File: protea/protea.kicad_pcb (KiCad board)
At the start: 2 copper layers, 92 x 44 mm, 72 parts, among them J1 USB4215-03-A, J2 D-SUB 9 Male, J3 676430910, J4 HDMI Female, J5 ESP8266 Prog, J6 SD04H0SB, U1 NCP1117 3.3, U2 W25Q128JVSIQ, U3 RP2040, U4 MAX232CSE+, U5 ESP8266-12E_ESP-12E, Y1 12 MHz

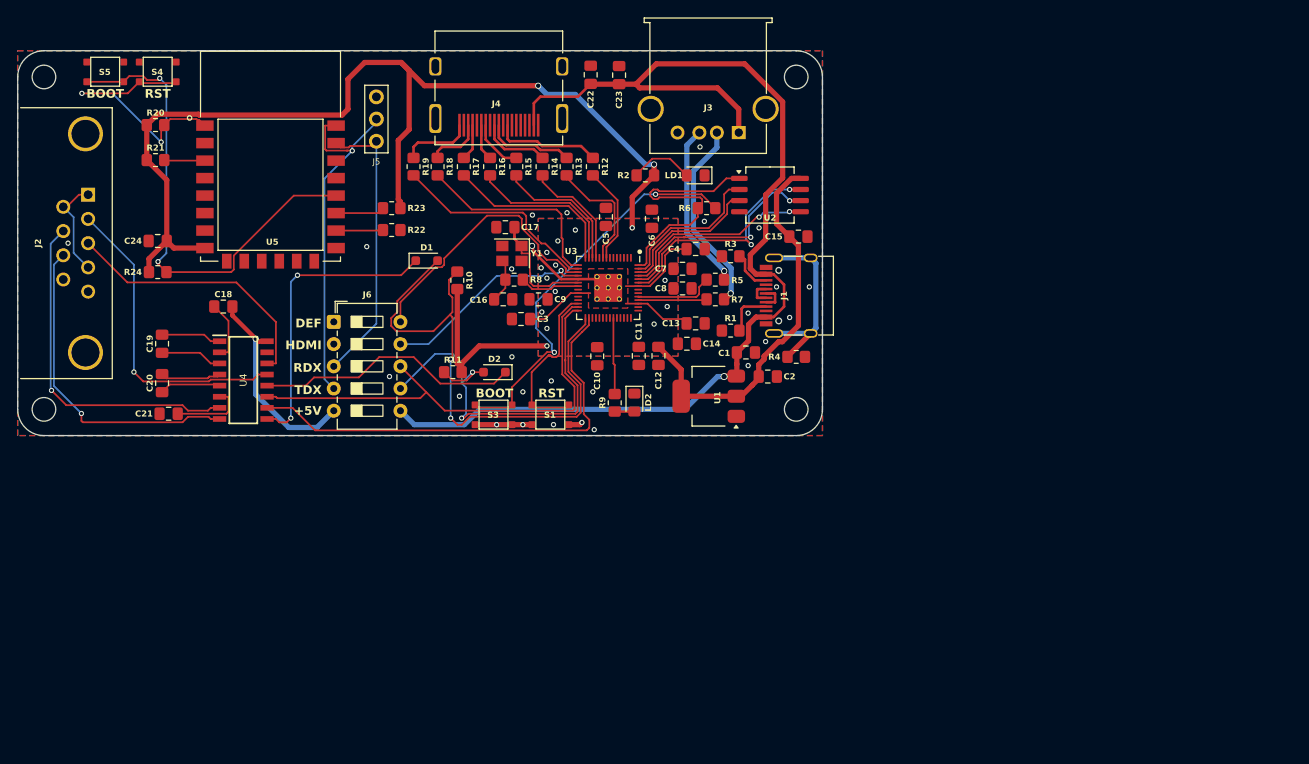
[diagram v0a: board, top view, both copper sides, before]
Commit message: Protea 1.1 WIP
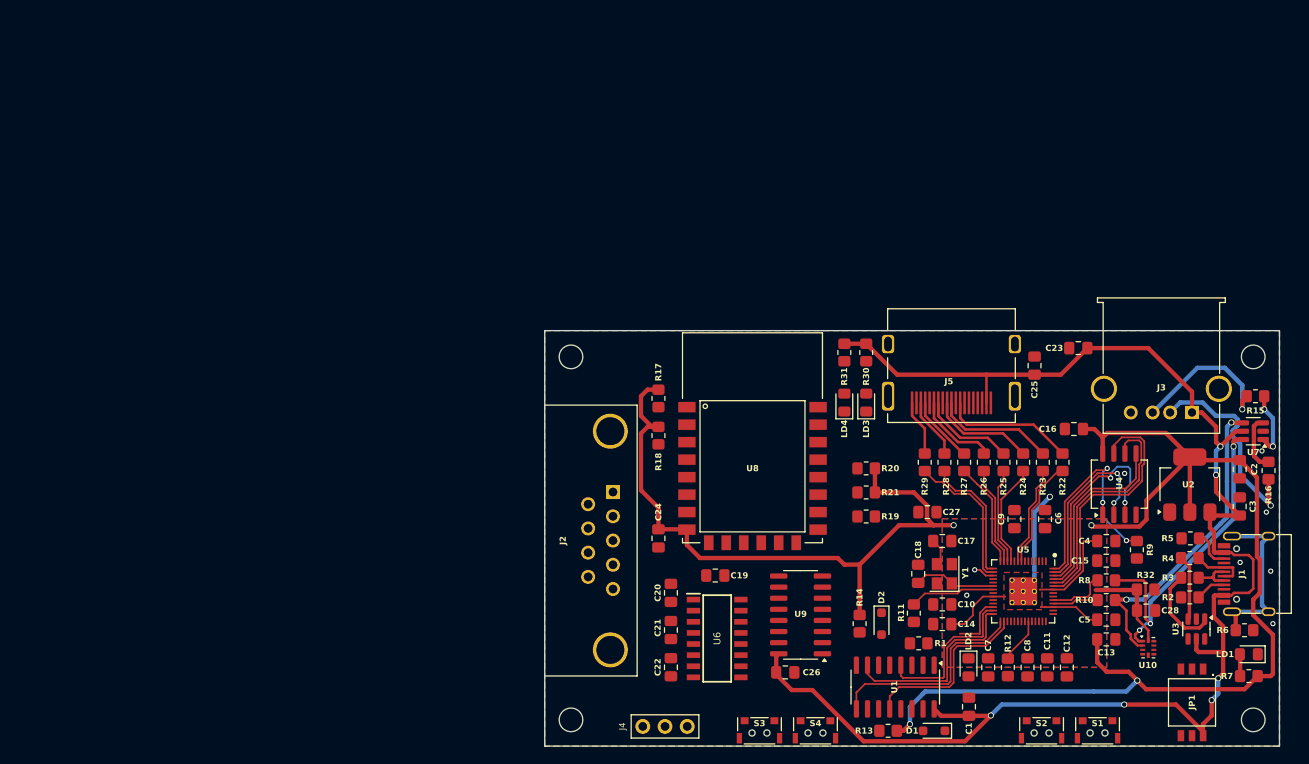
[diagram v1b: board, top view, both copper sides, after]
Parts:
- removed J6: SD04H0SB, FRANK:DIP Switch (5x5)
- removed S5: Flash, FRANK:Button (SMD, 3x3mm, 1-1)
- added C25: 100n, FRANK:Capacitor (0805), F.Cu at (193.8, 59.0)
- added C26: 100n, FRANK:Capacitor (0805), F.Cu at (165.2, 94.1)
- added C27: 100n, FRANK:Capacitor (0805), F.Cu at (181.5, 75.8)
- added C28: 100n, FRANK:Capacitor (0805), F.Cu at (206.5, 87.0)
- added JP1: Main Jumpers, FRANK:DS05127203BKSMTTR, F.Cu at (211.8, 97.5)
- added LD3: TX, FRANK:LED (0805), F.Cu at (174.5, 63.2)
- added LD4: RX, FRANK:LED (0805), F.Cu at (172.0, 63.2)
- added R25: 270R, FRANK:Resistor (0805), F.Cu at (190.2, 70.1)
- added R26: 270R, FRANK:Resistor (0805), F.Cu at (187.9, 70.1)
- added R27: 270R, FRANK:Resistor (0805), F.Cu at (185.7, 70.1)
- added R28: 270R, FRANK:Resistor (0805), F.Cu at (183.4, 70.1)
- added R29: 270R, FRANK:Resistor (0805), F.Cu at (181.2, 70.1)
- added R30: 1.5K, FRANK:Resistor (0805), F.Cu at (174.5, 57.5)
- added R31: 1.5K, FRANK:Resistor (0805), F.Cu at (172.0, 57.5)
- added R32: 10K, FRANK:Resistor (0805), F.Cu at (206.4, 84.6)
- added S2: Reset, FRANK:TACT-SIDE-4623, F.Cu at (194.6, 101.0)
- added U10: TS3USB221RSER, FRANK:UQFN-10, F.Cu at (206.8, 91.2)
- added U6: MAX232CSE+, FRANK:SOIC127P600X175-16N, F.Cu at (157.5, 90.2)
- added U7: USBLC6-2SC6, FRANK:SOT-23-6, F.Cu at (218.8, 66.5)
- added U8: ESP8266-12E_ESP-12E, FRANK:ESP8266 ESP-12E, F.Cu at (161.5, 70.8)
- added U9: CH340C, FRANK:SOP-16, F.Cu at (167.0, 87.5)
- C1: value 10u -> 100n
- C13: value 1u -> 100n
- C15: value 100n -> 1u
- C16: value 15p -> 100n
- C18: value 1u -> 15p
- C22: value 10u -> 1u
- C23, C3: value 100n -> 10u
- J4: value HDMI Female -> ESP8266 Prog; footprint FRANK:HDMI (female) -> FRANK:Pin Header (1x03)
- J5: value ESP8266 Prog -> HDMI Female; footprint FRANK:Pin Header (1x03) -> FRANK:HDMI (female)
- LD1: value Green -> Power
- R1: value 5.1K -> 10K
- R10, R8: value 1K -> 27R
- R12, R13, R14: value 270R -> 1K
- R15, R16: value 270R -> 22R
- R17, R18, R19: value 270R -> 10K
- R2: value 1K -> 5.1K
- R22, R23, R24: value 10K -> 270R
- R3: value 5.1K -> 22R
- R4: value 1M -> 22R
- R5: value 27R -> 5.1K
- R6: value 1K -> 1M
- R7: value 27R -> 1K
- S1: value Reset -> Boot; footprint FRANK:Button (SMD, 3x3mm, 1-1) -> FRANK:TACT-SIDE-4623
- S3: value Boot -> Reset; footprint FRANK:Button (SMD, 3x3mm, 1-1) -> FRANK:TACT-SIDE-4623
- S4: value Reset -> Flash; footprint FRANK:Button (SMD, 3x3mm, 1-1) -> FRANK:TACT-SIDE-4623
- U1: value NCP1117 3.3 -> SN74CBT3257CDR; footprint FRANK:SOT-223 -> FRANK:SOP-16
- U2: value W25Q128JVSIQ -> NCP1117 3.3; footprint FRANK:SOIC-8 -> FRANK:SOT-223
- U3: value RP2040 -> USBLC6-2SC6; footprint FRANK:QFN 56 -> FRANK:SOT-23-6
- U4: value MAX232CSE+ -> W25Q128JVSIQ; footprint FRANK:SOIC127P600X175-16N -> FRANK:SOIC-8
- U5: value ESP8266-12E_ESP-12E -> RP2040; footprint FRANK:ESP8266 ESP-12E -> FRANK:QFN 56
- moved H2 141.9 mm to (218.8, 58.0)
- moved S4 109.0 mm to (168.7, 101.0), turned to 180 degrees
- moved R24 101.3 mm to (192.4, 70.1), turned to -90 degrees
- moved U4 100.9 mm to (203.4, 72.6), turned to 90 degrees
- moved U5 97.7 mm to (192.4, 84.8), turned to -90 degrees
- moved R16 95.5 mm to (220.5, 71.0)
- moved R20 90.2 mm to (174.5, 70.8), turned to 180 degrees
- moved R21 89.7 mm to (174.5, 73.5), turned to 180 degrees
- moved R15 88.5 mm to (219.0, 62.5), turned to 180 degrees
- moved C18 85.1 mm to (180.4, 82.8), turned to 90 degrees
- moved C3 84.9 mm to (217.2, 75.1), turned to 90 degrees
- moved LD1 83.7 mm to (218.2, 92.0)
- moved R10 82.7 mm to (201.9, 85.8), turned to 180 degrees
- moved R22 81.2 mm to (196.9, 70.1), turned to -90 degrees
- moved R23 79.9 mm to (194.7, 70.1), turned to -90 degrees
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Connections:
- C1 pad 1: VBUS -> GND
- C1 pad 2: GND -> VBUS
- C13 pad 1: Net-(U3-VREG_VOUT) -> +3V3
- C14 pad 1: +3V3 -> Net-(U5-VREG_VOUT)
- C16 pad 1: Net-(C16-Pad1) -> +3V3
- C17 pad 1: /RP2040/XIN -> Net-(C17-Pad1)
- C18 pad 1: /RS232/V+ -> /RP2040/XIN
- C18 pad 2: /RS232_VBUS -> GND
- C19 pad 1: /RS232/C1- -> /RS232/V+
- C19 pad 2: /RS232/C1+ -> /RS232_VBUS
- C20 pad 1: /RS232/C2- -> /RS232/C1-
- C20 pad 2: /RS232/C2+ -> /RS232/C1+
- C21 pad 1: /RS232/V- -> /RS232/C2-
- C21 pad 2: GND -> /RS232/C2+
- C22 pad 1: GND -> /RS232/V-
- C22 pad 2: VBUS -> GND
- C23 pad 1: VBUS -> GND
- C23 pad 2: GND -> VBUS
- C3 pad 1: Net-(U3-VREG_VOUT) -> VBUS
- C4 pad 1: Net-(U3-VREG_VOUT) -> Net-(U5-VREG_VOUT)
- C5 pad 1: +3V3 -> Net-(U5-VREG_VOUT)
- D1 pad 2: /GPIO18 -> /RS232_CTS
- D2 pad 2: /GPIO17 -> /RS232_RX
- J1 pad 5: /Power/D- -> Net-(J1-DN1)
- J1 pad 6: /Power/D+ -> Net-(J1-DP1)
- J1 pad 7: /Power/D- -> Net-(J1-DN1)
- J1 pad 8: /Power/D+ -> Net-(J1-DP1)
- J3 pad 2: /D- -> Net-(J3-D-)
- J3 pad 3: /D+ -> Net-(J3-D+)
- J4 pad 1: Net-(J4-D2P) -> /ESP_RXD
- J4 pad 2: GND -> /ESP_TXD
- J4 pad 3: Net-(J4-D2N) -> GND
- J5 pad 1: /ESP_RXD -> Net-(J5-D2P)
- J5 pad 2: /ESP_TXD -> GND
- J5 pad 3: GND -> Net-(J5-D2N)
- R1 pad 2: Net-(J1-CC1) -> /SN74_S
- R10 pad 1: /GPIO18 -> /RP_D-
- R10 pad 2: +3V3 -> Net-(U5-USB_DM)
- R11 pad 1: /GPIO17 -> /RP2040/XOUT
- R11 pad 2: +3V3 -> Net-(C17-Pad1)
- R12 pad 1: Net-(J4-CLKN) -> Net-(LD2-A)
- R12 pad 2: /GPIO6 -> /RP2040/GPIO25
- R13 pad 1: Net-(J4-CLKP) -> /RS232_CTS
- R13 pad 2: /GPIO7 -> +3V3
- R14 pad 1: Net-(J4-D0N) -> /RS232_RX
- R14 pad 2: /GPIO8 -> +3V3
- R15 pad 1: Net-(J4-D0P) -> Net-(R15-Pad1)
- R15 pad 2: /GPIO9 -> Net-(J3-D+)
- R16 pad 1: Net-(J4-D1N) -> Net-(R16-Pad1)
- R16 pad 2: /GPIO10 -> Net-(J3-D-)
- R17 pad 1: Net-(J4-D1P) -> +3V3
- R17 pad 2: /GPIO11 -> Net-(U8-RESET)
- R18 pad 1: Net-(J4-D2N) -> +3V3
- R18 pad 2: /GPIO12 -> Net-(U8-EN)
- R19 pad 1: Net-(J4-D2P) -> GND
- R19 pad 2: /GPIO13 -> Net-(U8-IO15)
- R2 pad 1: Net-(LD1-A) -> GND
- R2 pad 2: +3V3 -> Net-(J1-CC1)
- R20 pad 2: Net-(U5-RESET) -> Net-(U8-IO0)
- R21 pad 2: Net-(U5-EN) -> Net-(U8-IO2)
- R22 pad 1: GND -> Net-(J5-CLKN)
- R22 pad 2: Net-(U5-IO15) -> /GPIO6
- R23 pad 1: +3V3 -> Net-(J5-CLKP)
- R23 pad 2: Net-(U5-IO2) -> /GPIO7
- R24 pad 1: +3V3 -> Net-(J5-D0N)
- R24 pad 2: Net-(U5-IO0) -> /GPIO8
- R3 pad 1: GND -> Net-(R3-Pad1)
- R3 pad 2: Net-(J1-CC2) -> Net-(J1-DN1)
- R4 pad 1: Net-(J1-SHIELD) -> Net-(R4-Pad1)
- R4 pad 2: GND -> Net-(J1-DP1)
- R5 pad 1: /D+ -> GND
- R5 pad 2: Net-(U3-USB_DP) -> Net-(J1-CC2)
- R6 pad 1: /RP2040/QSPI_SS -> Net-(J1-SHIELD)
- R6 pad 2: Net-(R6-Pad2) -> GND
- R7 pad 1: /D- -> Net-(LD1-A)
- R7 pad 2: Net-(U3-USB_DM) -> +3V3
- R8 pad 1: /RP2040/XOUT -> /RP_D+
- R8 pad 2: Net-(C16-Pad1) -> Net-(U5-USB_DP)
- R9 pad 1: Net-(LD2-A) -> /RP2040/QSPI_SS
- R9 pad 2: /RP2040/GPIO25 -> Net-(R9-Pad2)
- S1 pad 1: /RUN -> Net-(R9-Pad2)
- S3 pad 1: Net-(R6-Pad2) -> GND
- S3 pad 2: GND -> Net-(U8-RESET)
- S4 pad 2: Net-(U5-RESET) -> Net-(U8-IO0)
- U1 pad 1: GND -> /SN74_S
- U1 pad 2: +3V3 -> /ESP_RXD
- U1 pad 3: VBUS -> /RS232_TX
- U2 pad 1: /RP2040/QSPI_SS -> GND
- U2 pad 2: /RP2040/QSPI_SD1 -> +3V3
- U2 pad 3: /RP2040/QSPI_SD2 -> VBUS
- U3 pad 1: +3V3 -> Net-(R3-Pad1)
- U3 pad 2: /GPIO0 -> GND
- U3 pad 3: /GPIO1 -> Net-(R4-Pad1)
- U3 pad 4: /GPIO2 -> /PW_D+
- U3 pad 5: /GPIO3 -> VBUS
- U3 pad 6: /GPIO4 -> /PW_D-
- U4 pad 1: /RS232/C1+ -> /RP2040/QSPI_SS
- U4 pad 2: /RS232/V+ -> /RP2040/QSPI_SD1
- U4 pad 3: /RS232/C1- -> /RP2040/QSPI_SD2
- U4 pad 4: /RS232/C2+ -> GND
- U4 pad 5: /RS232/C2- -> /RP2040/QSPI_SD0
- U4 pad 6: /RS232/V- -> /RP2040/QSPI_SCLK
- U4 pad 7: /RS232/CTS_IN -> /RP2040/QSPI_SD3
- U4 pad 8: /RS232/RTS_IN -> +3V3
- U5 pad 1: Net-(U5-RESET) -> +3V3
- U5 pad 10: /ESP_MISO -> +3V3
- U5 pad 11: /ESP_GPIO9 -> /GPIO8
- U5 pad 12: /ESP_GPIO10 -> /GPIO9
- U5 pad 13: /ESP_MOSI -> /GPIO10
- U5 pad 14: /ESP_SCLK -> /GPIO11
- U5 pad 15: GND -> /GPIO12
- U5 pad 16: Net-(U5-IO15) -> /GPIO13
- U5 pad 17: Net-(U5-IO2) -> /GPIO14
- U5 pad 18: Net-(U5-IO0) -> /GPIO15
- U5 pad 19: /ESP_GPIO4 -> GND
- U5 pad 2: /ESP_ADC -> /GPIO0
- U5 pad 20: /ESP_GPIO5 -> /RP2040/XIN
- U5 pad 21: /ESP_RXD -> /RP2040/XOUT
- U5 pad 22: /ESP_TXD -> +3V3
- U5 pad 3: Net-(U5-EN) -> /GPIO1
- U5 pad 4: /ESP_GPIO16 -> /GPIO2
- U5 pad 5: /ESP_GPIO14 -> /GPIO3
- U5 pad 6: /ESP_GPIO12 -> /GPIO4
- U5 pad 7: /ESP_GPIO13 -> /GPIO5
- U5 pad 8: +3V3 -> /GPIO6
- U5 pad 9: /ESP_CSO -> /GPIO7
- Y1 pad 3: Net-(C16-Pad1) -> Net-(C17-Pad1)
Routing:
- net Net-(U5-IO0): track 56.1 -> 0.00 mm, vias 2 -> 0
- net Net-(R6-Pad2): track 45.9 -> 0.00 mm, vias 2 -> 0
- net VBUS: track 132.1 -> 176.4 mm, vias 1 -> 6
- net /ESP_TXD: track 40.8 -> 0.00 mm, vias 1 -> 0
- net /RS232/CTS_IN: track 39.2 -> 0.00 mm, vias 1 -> 0
- net /GPIO18: track 63.0 -> 24.3 mm, vias 2 -> 0
- net /RP_D+: track 0.00 -> 38.1 mm, vias 0 -> 3
- net /RS232/RTS_IN: track 36.9 -> 0.00 mm, vias 1 -> 0
- net /RP_D-: track 0.00 -> 36.1 mm, vias 0 -> 2
- net /RS232/TX_IN: track 35.7 -> 0.00 mm, vias 1 -> 0
- net /GPIO16: track 54.1 -> 18.6 mm
- net /RS232/CTS_MAX: track 33.9 -> 0.00 mm, vias 2 -> 0
- net /ESP_RXD: track 32.8 -> 0.00 mm
- net /GPIO19: track 52.3 -> 20.7 mm
- net /RS232/RX_IN: track 31.0 -> 0.00 mm
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- added copper zone on F.Cu, net Net-(U5-VREG_VOUT)
- removed copper zone on F.Cu, net Net-(U3-VREG_VOUT)
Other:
- board size 92 x 44 mm -> 84 x 47.5 mm
- board text removed: "${VERSION}"
- board text removed: "+5V"
- board text removed: "BOOT"
- board text removed: "DEF"
- board text removed: "HDMI"
- board text removed: "Protea"
- board text removed: "RDX"
- board text removed: "RST"
- board text removed: "TDX"
- board text removed: "rh1.tech"
